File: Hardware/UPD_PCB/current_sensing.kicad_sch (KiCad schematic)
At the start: 60 parts, among them Q6 BSS84, U1 INA228, U2 INA228, U3 INA228, U4 INA228, U5 ACS711xEXLT-31AB, U6 INA228

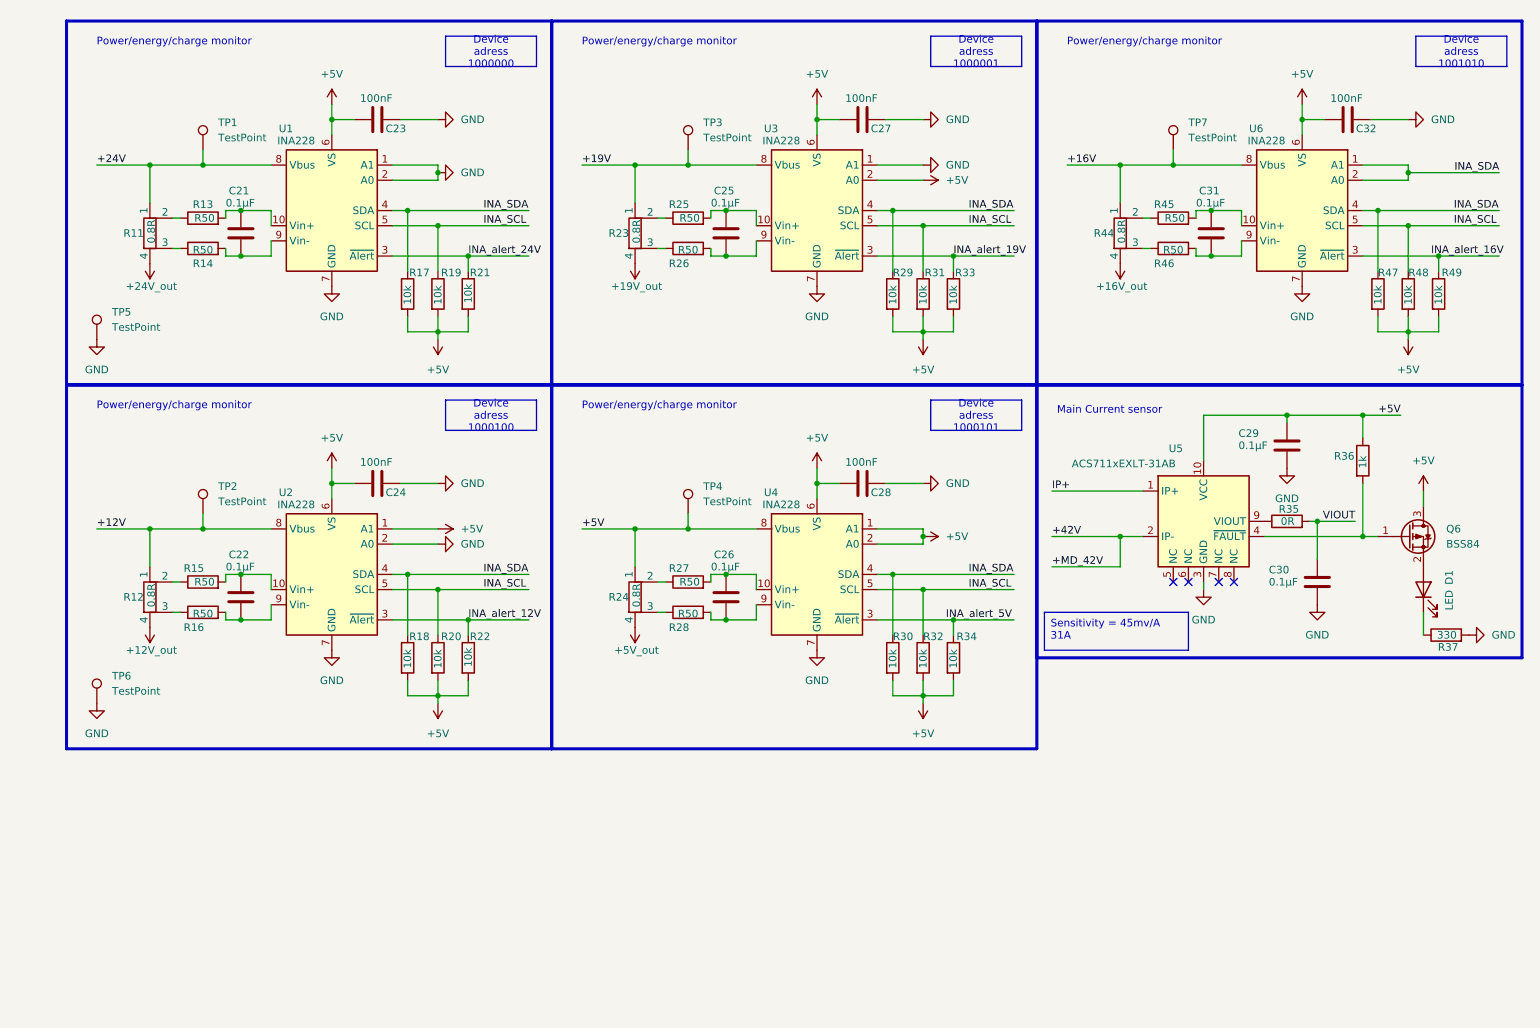
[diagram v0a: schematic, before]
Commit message: Finalized Schematic
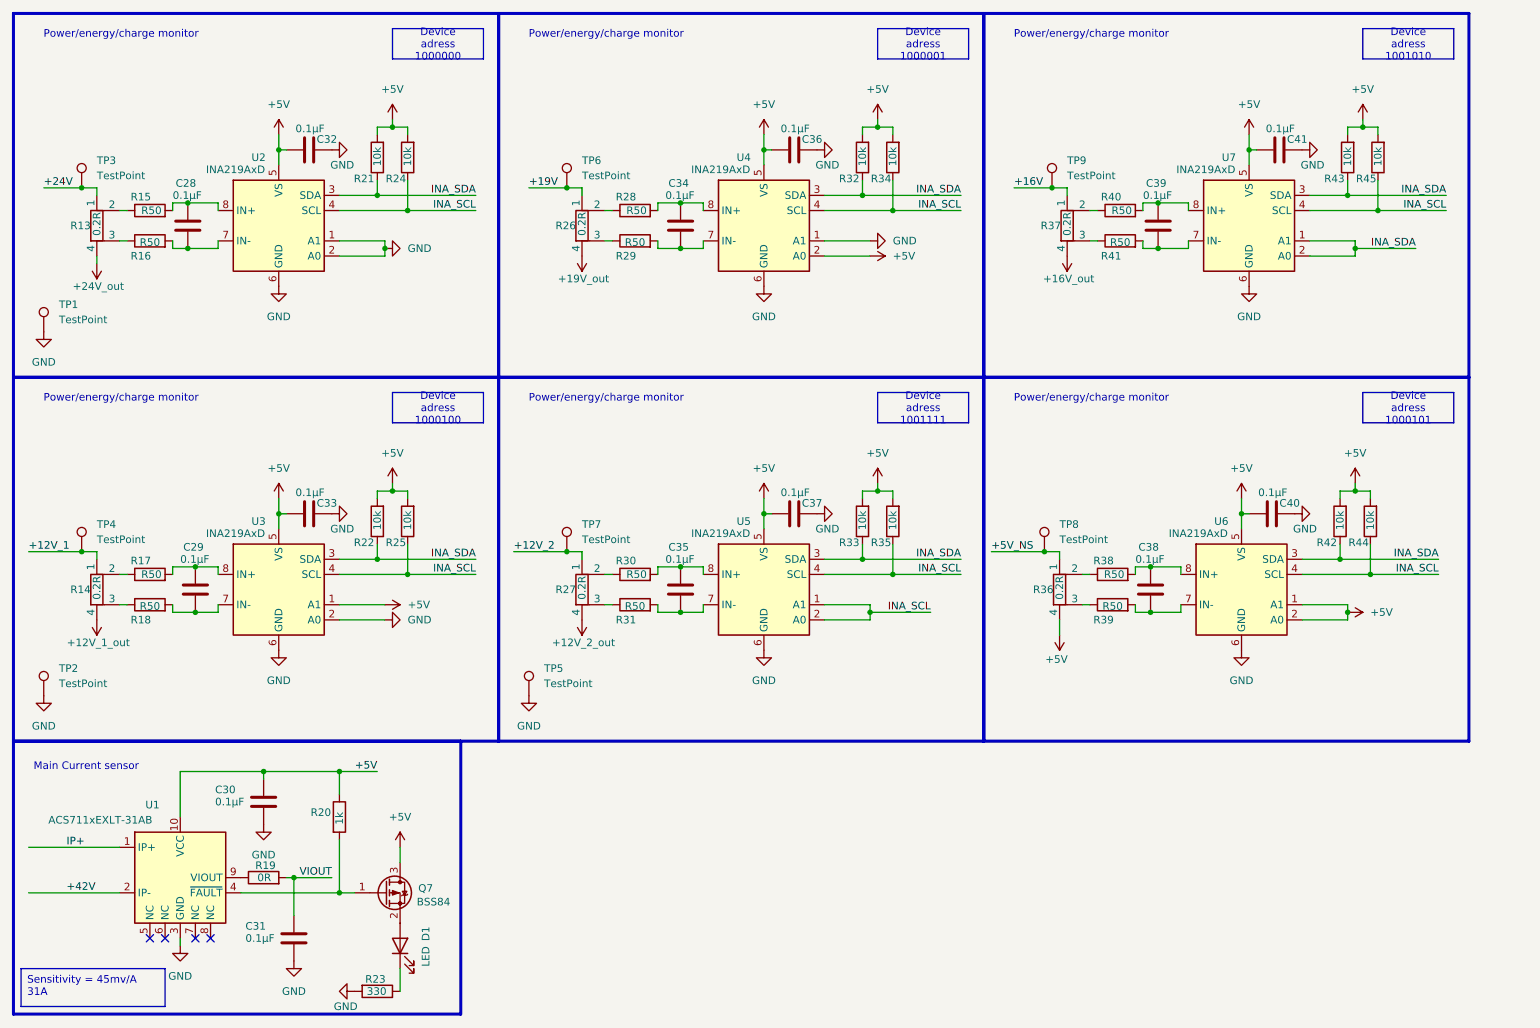
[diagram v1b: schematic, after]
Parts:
- removed C21, C22, C25, C26, C31: 0.1µF, symbol Device:C
- removed C23, C24, C27: 100nF, Capacitor_SMD:C_0603_1608Metric_Pad1.08x0.95mm_HandSolder, symbol Device:C
- removed R11, R12, R23, R24, R44: 0.8R, Resistor_SMD:R_2512_6332Metric_Pad1.40x3.35mm_HandSolder, symbol Device:R_Shunt
- removed R13, R14, R26, R27, R46: R50, Resistor_SMD:R_0603_1608Metric_Pad0.98x0.95mm_HandSolder, symbol Device:R
- removed R19, R20, R47, R48, R49: 10k, Resistor_SMD:R_0603_1608Metric_Pad0.98x0.95mm_HandSolder, symbol Device:R
- removed TP1, TP2: TestPoint, TestPoint:TestPoint_Loop_D2.54mm_Drill1.5mm_Beaded, symbol Connector:TestPoint
- removed U1, U2, U3, U4, U6: INA228, Package_SO:VSSOP-10_3x3mm_P0.5mm, symbol Sensor_Energy:INA228
- added C29, C33, C34, C35, C36, C37, C38, C39, C40, C41: 0.1µF, Capacitor_SMD:C_0603_1608Metric_Pad1.08x0.95mm_HandSolder, symbol Device:C
- added R13, R14, R26, R27, R36, R37: 0.2R, Resistor_SMD:R_Shunt_Vishay_WSK2512_6332Metric_T2.21mm, symbol Device:R_Shunt
- added R24, R35, R42, R43, R44: 10k, Resistor_SMD:R_0603_1608Metric_Pad0.98x0.95mm_HandSolder, symbol Device:R
- added R38, R39, R40, R41: R50, Resistor_SMD:R_0603_1608Metric_Pad0.98x0.95mm_HandSolder, symbol Device:R
- added TP5, TP6, TP8, TP9: TestPoint, TestPoint:TestPoint_Loop_D2.54mm_Drill1.5mm_Beaded, symbol Connector:TestPoint
- added U2, U3, U4, U5, U6, U7: INA219AxD, Package_SO:SOIC-8_3.9x4.9mm_P1.27mm, symbol Sensor_Energy:INA219AxD
- C28, C32: value 100nF -> 0.1µF
- R17, R18, R29, R30, R31: value 10k -> R50
- R25, R45: value R50 -> 10k
- renumbered C29 to C30, C30 to C31, Q6 to Q7, R35 to R19, R36 to R20, R37 to R23, TP5 to TP1, TP6 to TP2, U5 to U1
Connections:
- net INA_alert_12V is gone; now on net INA_SDA: R22.1
- net INA_alert_19V is gone; now on net INA_SDA: R33.1
- net INA_alert_24V is gone; now on net INA_SDA: R21.1
- net INA_alert_5V is gone; now on net INA_SCL: R34.1
- net +16V: now also R37.1, TP9.1; no longer TP7.1
- net +16V_out: now also R37.4
- net +19V: now also R26.1, TP6.1; no longer TP3.1
- net +19V_out: now also R26.4
- net +24V: now also TP3.1, R13.1
- net +24V_out: now also R13.4
- net +5V: now also C32.2, R25.2, R45.2, C33.2, C36.2, C37.2, C40.2, C41.2, R24.2, R35.2, R36.4, R42.2, R43.2, R44.2, U2.5 (VS), U3.1 (A1), U3.5 (VS), U4.2 (A0), U4.5 (VS), U5.5 (VS), U6.1 (A1), U6.2 (A0), U6.5 (VS), U7.5 (VS); no longer C28.1, C32.1, R17.2, R18.2, R29.2, R30.2, R31.2, TP4.1
- net GND: now also C32.1, C33.1, C36.1, C37.1, C40.1, C41.1, TP5.1, U2.1 (A1), U2.2 (A0), U2.6 (GND), U3.2 (A0), U3.6 (GND), U4.1 (A1), U4.6 (GND), U5.6 (GND), U6.6 (GND), U7.6 (GND); no longer C28.2, C32.2
- net INA_SCL: now also R25.1, R45.1, R24.1, R35.1, R44.1, U2.4 (SCL), U3.4 (SCL), U4.4 (SCL), U5.1 (A1), U5.2 (A0), U5.4 (SCL), U6.4 (SCL), U7.4 (SCL); no longer R31.1, R32.1
- net INA_SDA: now also R32.1, R42.1, R43.1, U2.3 (SDA), U3.3 (SDA), U4.3 (SDA), U5.3 (SDA), U6.3 (SDA), U7.1 (A1), U7.2 (A0), U7.3 (SDA); no longer R17.1, R18.1, R29.1, R30.1
- net at R28.1: now also R26.2
- net at R28.2: now also C34.1, U4.8 (IN+)
- net at R15.1: now also R13.2
- net at R15.2: now also C28.1, U2.8 (IN+)
- net at R16.2: now also C28.2, U2.7 (IN-)
- net at R16.1: now also R13.3
- new net: C39.1, R40.2, U7.8 (IN+)
- new net: C39.2, R41.2, U7.7 (IN-)
- new net: C38.2, R39.2, U6.7 (IN-)
- new net: C38.1, R38.2, U6.8 (IN+)
- new net: R27.2, R30.1
- new net: R27.3, R31.1
- new net: R26.3, R29.1
- new net: C34.2, R29.2, U4.7 (IN-)
- new net: C35.1, R30.2, U5.8 (IN+)
- new net: R36.2, R38.1
- new net: R37.3, R41.1
- new net: C35.2, R31.2, U5.7 (IN-)
- new net: R37.2, R40.1
- new net: R14.2, R17.1
- new net: R14.3, R18.1
- new net: C29.1, R17.2, U3.8 (IN+)
- new net: R36.3, R39.1
- new net: C29.2, R18.2, U3.7 (IN-)
- new net +12V_1: R14.1, TP4.1
- new net +12V_1_out: R14.4
- new net +12V_2: R27.1, TP7.1
- new net +12V_2_out: R27.4
- new net +5V_NS: R36.1, TP8.1
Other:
- moved on the sheet: C30, C31, D1, Q7, R19, R20, R23, TP1, TP2, U1
